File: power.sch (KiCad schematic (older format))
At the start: 8 parts, among them U1 4070, U2 40106, U3 LM358

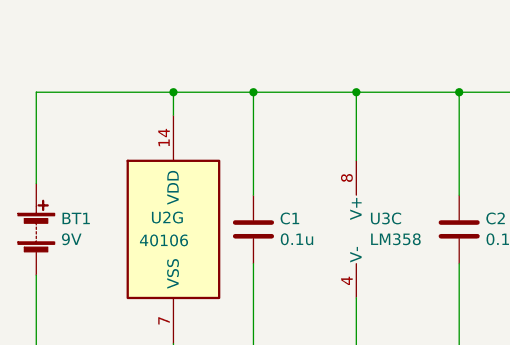
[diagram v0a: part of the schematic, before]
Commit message: Small changes to the Schematics for readability More docs Add abstract for Booster
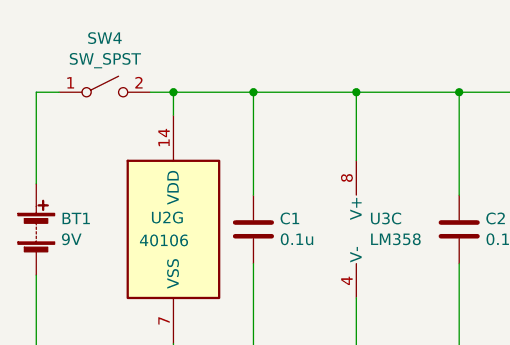
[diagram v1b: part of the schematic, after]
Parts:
- added SW4: SW_SPST, symbol Switch:SW_SPST
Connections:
- net +9V: now also SW4.2 (B); no longer BT1.1 (+)
- new net: BT1.1 (+), SW4.1 (A)
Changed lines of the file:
@@
 $Descr A4 11693 8268
 encoding utf-8
-Sheet 2 8
+Sheet 2 7
 Title ""
 Date ""
@@
 	5400 2300 5400 2400
 Wire Wire Line
-	1500 1400 2100 1400
+	1500 1400 1600 1400
 Wire Wire Line
 	1500 2600 2100 2600
@@
 Wire Wire Line
 	4300 2600 4800 2600
+$Comp
+L Switch:SW_SPST SW4
+U 1 1 5E203D92
+P 1800 1400
+F 0 "SW4" H 1800 1635 50  0000 C CNN
+F 1 "SW_SPST" H 1800 1544 50  0000 C CNN
+F 2 "" H 1800 1400 50  0001 C CNN
+F 3 "~" H 1800 1400 50  0001 C CNN
+	1    1800 1400
+	1    0    0    -1
+$EndComp
+Wire Wire Line
+	2000 1400 2100 1400
 $EndSCHEMATC
